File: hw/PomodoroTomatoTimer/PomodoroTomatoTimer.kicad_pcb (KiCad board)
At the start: 2 copper layers, 25.4 x 25.4 mm, 19 parts, among them J1 Coin Cell, SW1 SW_DIP_x02, U1 STM32F030F4Px

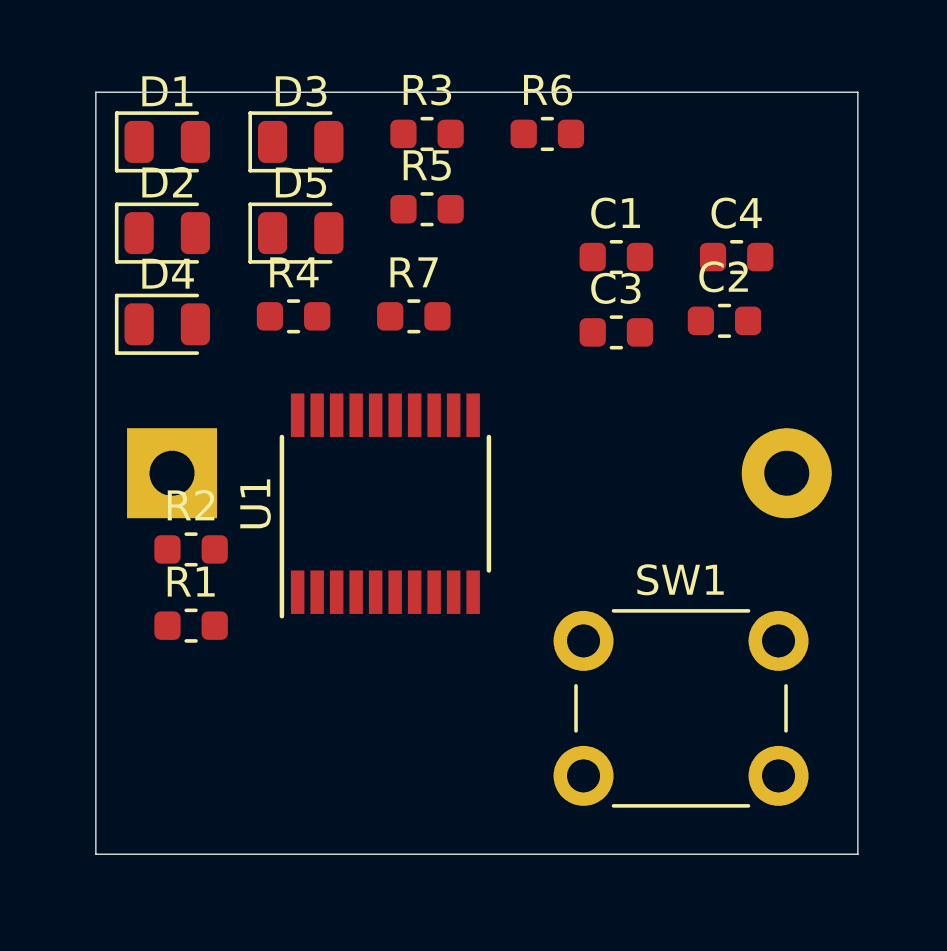
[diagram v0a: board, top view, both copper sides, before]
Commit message: + Placement and routing ok.
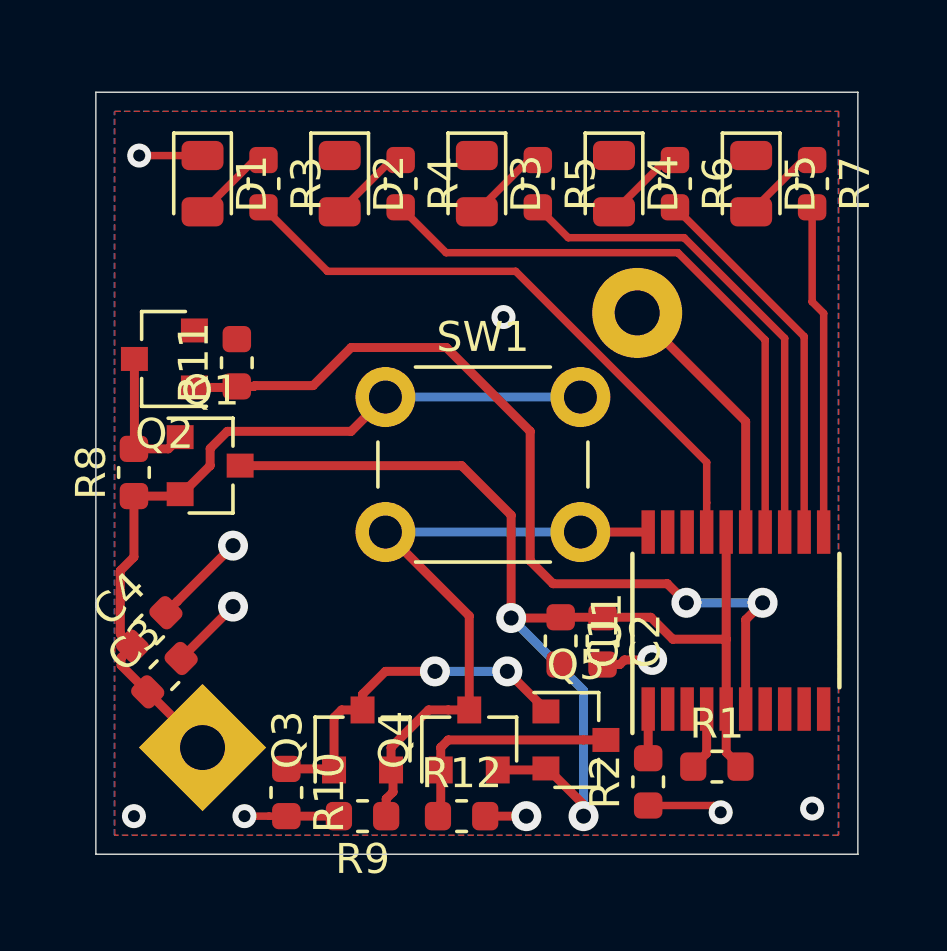
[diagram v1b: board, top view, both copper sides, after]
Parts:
- added Q1: BSS83P, Package_TO_SOT_SMD:SOT-23, F.Cu at (130.8, 88.6)
- added Q2: 2N7002, Package_TO_SOT_SMD:SOT-23, F.Cu at (129.3, 85.1)
- added Q3: BC807, Package_TO_SOT_SMD:SOT-23, F.Cu at (135.9, 97.8)
- added Q4: BSS83P, Package_TO_SOT_SMD:SOT-23, F.Cu at (139.4, 97.8)
- added Q5: BC807, Package_TO_SOT_SMD:SOT-23, F.Cu at (143.0, 97.8)
- added R10: 47k 0603, Resistor_SMD:R_0603_1608Metric, F.Cu at (133.3, 99.5)
- added R11: 10k 0603, Resistor_SMD:R_0603_1608Metric, F.Cu at (131.7, 85.2)
- added R12: 47k 0603, Resistor_SMD:R_0603_1608Metric, F.Cu at (139.2, 100.3)
- added R8: 10k 0603, Resistor_SMD:R_0603_1608Metric, F.Cu at (128.3, 88.9)
- added R9: 10k 0603, Resistor_SMD:R_0603_1608Metric, F.Cu at (135.9, 100.3)
- SW1: value SW_DIP_x02 -> SW_DPST_x2
- moved C4 23.2 mm to (128.8, 94.1), turned to 45 degrees
- moved C3 18.9 mm to (129.3, 95.6), turned to 45 degrees
- moved R1 18.1 mm to (147.7, 98.7)
- moved R2 17.1 mm to (145.4, 99.2), turned to 90 degrees
- moved D4 15.6 mm to (144.3, 79.2), turned to 270 degrees
- moved D5 15.1 mm to (148.8, 79.2), turned to 270 degrees
- moved R7 14.0 mm to (150.9, 79.2), turned to 270 degrees
- moved C1 12.9 mm to (142.5, 94.5), turned to 270 degrees
- moved U1 12.3 mm to (148.3, 93.8)
- moved C2 11.4 mm to (143.9, 94.5), turned to 270 degrees
- moved SW1 10.5 mm to (136.7, 86.4)
- moved J1 9.20 mm to (130.6, 98.0), turned to 45 degrees
- moved D3 6.03 mm to (139.7, 79.2), turned to 270 degrees
- moved D2 5.98 mm to (135.1, 79.2), turned to 270 degrees
- moved R3 5.70 mm to (132.6, 79.2), turned to 270 degrees
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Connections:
- SW1 pad 1: Net-(SW1-Pad1) -> VDDA
- SW1 pad 2: Net-(SW1-Pad2) -> /BUTTON
- U1 pad 11: Net-(U1-Pad11) -> /LED5
- U1 pad 12: Net-(U1-Pad12) -> /LED4
- U1 pad 13: Net-(U1-Pad13) -> /LED3
- U1 pad 14: Net-(U1-Pad14) -> /LED2
- U1 pad 17: Net-(U1-Pad17) -> /LED1
- U1 pad 20: Net-(U1-Pad20) -> /BUTTON
- U1 pad 6: Net-(U1-Pad6) -> /POW_CTRL
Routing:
- net VDD: track 0.00 -> 40.0 mm, vias 0 -> 2
- net /POW_CTRL: track 0.00 -> 29.3 mm, vias 0 -> 2
- net VDDA: track 0.00 -> 26.6 mm
- net GND: track 0.00 -> 25.3 mm, vias 0 -> 10
- net /BUTTON: track 0.00 -> 21.4 mm
- net /LED1: track 0.00 -> 20.6 mm
- net /LED2: track 0.00 -> 20.4 mm
- net /LED3: track 0.00 -> 16.5 mm
- net /LED4: track 0.00 -> 12.6 mm
- net Net-(Q3-Pad1): track 0.00 -> 11.9 mm, vias 0 -> 2
- net /LED5: track 0.00 -> 11.0 mm
- net Net-(Q4-Pad1): track 0.00 -> 7.94 mm
- net Net-(Q1-Pad1): track 0.00 -> 4.71 mm
- net Net-(D5-Pad2): track 0.00 -> 2.75 mm
- net Net-(D4-Pad2): track 0.00 -> 2.75 mm
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- added copper zone on B.Cu, net GND
- added copper zone on F.Cu, net GND
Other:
- net class Default: clearance 0.2 -> 0.25
- rule trace_clearance: 0.2 -> 0.25
